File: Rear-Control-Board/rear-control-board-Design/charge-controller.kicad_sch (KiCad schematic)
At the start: 2 parts

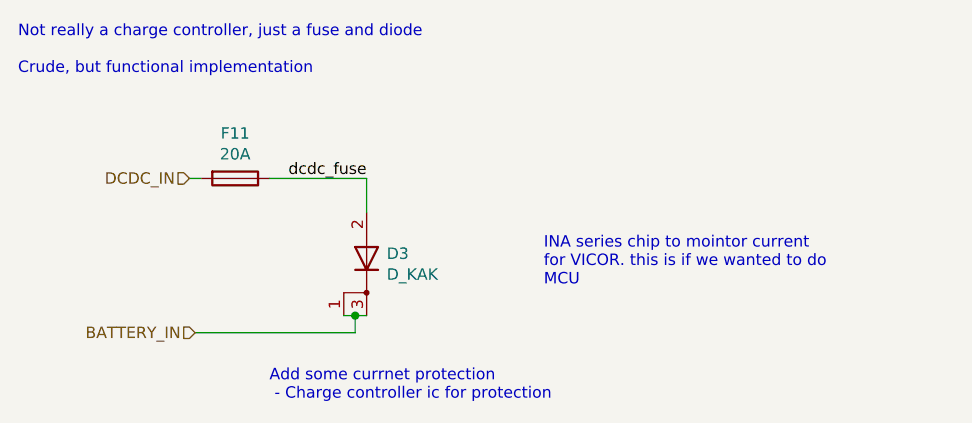
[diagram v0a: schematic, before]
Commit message: pcb Done? check SD
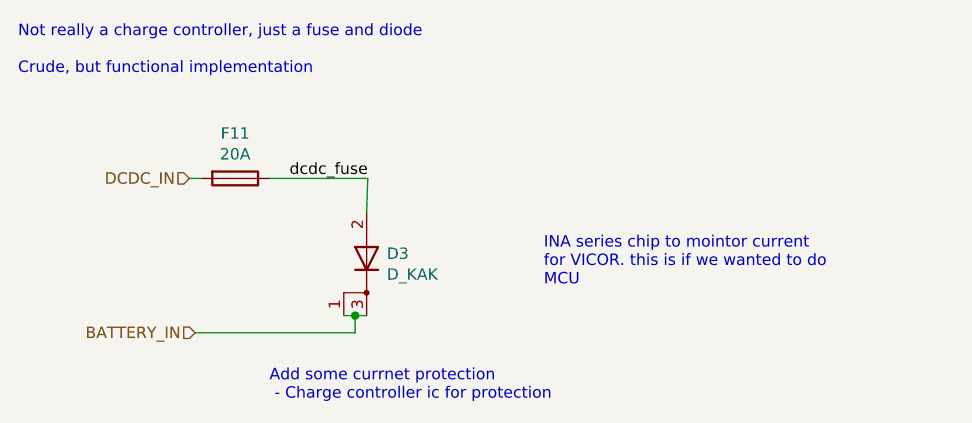
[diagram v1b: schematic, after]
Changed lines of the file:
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@@
   (junction (at 117.475 97.79) (diameter 0) (color 0 0 0 0)
   )
-  (wire (pts (xy 107.95 82.55) (xy 118.745 82.55))
+  (wire (pts (xy 107.95 82.55) (xy 118.872 82.55))
     (stroke (width 0) (type default) (color 0 0 0 0))
   )
@@
     (stroke (width 0) (type default) (color 0 0 0 0))
   )
-  (wire (pts (xy 118.745 82.55) (xy 118.745 86.36))
+  (wire (pts (xy 118.872 82.55) (xy 118.745 86.36))
     (stroke (width 0) (type default) (color 0 0 0 0))
   )
@@
     (effects (font (size 1.27 1.27)) (justify left bottom))
   )
-  (label "dcdc_fuse" (at 118.745 82.55 180)
+  (label "dcdc_fuse" (at 118.872 82.55 180)
     (effects (font (size 1.27 1.27)) (justify right bottom))
   )
